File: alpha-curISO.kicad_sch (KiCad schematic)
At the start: 169 parts, among them SW1 SW_Push_45deg, SW10 SW_Push_45deg, SW11 SW_Push_45deg, SW11(2)1 SW_Push_45deg, SW12 SW_Push_45deg, SW13 SW_Push_45deg, SW14 SW_Push_45deg, SW15 SW_Push_45deg, SW16 SW_Push_45deg, SW17 SW_Push_45deg, SW18 SW_Push_45deg, SW19 SW_Push_45deg, SW2 SW_Push_45deg, SW20 SW_Push_45deg, SW21 SW_Push_45deg, SW22 SW_Push_45deg, SW22(1.5)1 SW_Push_45deg, SW23 SW_Push_45deg, SW23(1.5)1 SW_Push_45deg, SW24 SW_Push_45deg, SW24(2)1 SW_Push_45deg, SW24(ISO)1 SW_Push_45deg, SW25 SW_PUSH, SW25(1.25)1 SW_Push_45deg, SW25(1.5)1 SW_Push_45deg, SW25(ortho)1 SW_Push_45deg, SW26 SW_Push_45deg, SW26(ortho)1 SW_Push_45deg, SW27 SW_Push_45deg, SW27(ortho)1 SW_Push_45deg, SW28 SW_Push_45deg, SW28(ortho)1 SW_Push_45deg, SW29 SW_Push_45deg, SW29(ortho)1 SW_Push_45deg, SW3 SW_Push_45deg, SW30 SW_Push_45deg, SW30(ortho)1 SW_Push_45deg, SW31 SW_Push_45deg, SW31(ortho)1 SW_Push_45deg, SW32 SW_Push_45deg, SW32(ortho)1 SW_Push_45deg, SW33 SW_Push_45deg, SW33(ortho)1 SW_Push_45deg, SW34 SW_Push_45deg, SW34(ortho)1 SW_Push_45deg, SW35 SW_Push_45deg, SW35(ortho)1 SW_Push_45deg, SW36 SW_PUSH, SW36(1.25)1 SW_Push_45deg, SW36(1.5)1 SW_Push_45deg, SW36(ortho)1 SW_Push_45deg, SW37 SW_Push_45deg, SW37(1.5)1 SW_Push_45deg, SW38 SW_Push_45deg, SW38(3)1 SW_Push_45deg, SW39 SW_Push_45deg, SW39(1.5)1 SW_Push_45deg, SW4 SW_Push_45deg, SW40 SW_PUSH, SW40(1.25)1 SW_Push_45deg, SW40(1.5)1 SW_Push_45deg, SW40(3)1 SW_Push_45deg, SW41(1.75)1 SW_Push_45deg, SW41(1.75a)1 SW_Push_45deg, SW41(1.75a)2 SW_Push_45deg, SW41(2)1 SW_Push_45deg, SW41(2.25)1 SW_Push_45deg, SW42 SW_Push_45deg, SW42(3)1 SW_Push_45deg, SW42(6)1 SW_Push_45deg, SW43(1.75)1 SW_Push_45deg, SW43(2)1 SW_Push_45deg, SW43(2.25)1 SW_Push_45deg, SW44(1.25)1 SW_Push_45deg, SW44(1.5)1 SW_Push_45deg, SW44(3)1 SW_Push_45deg, SW45 SW_Push_45deg, SW45(1.5)1 SW_Push_45deg, SW46 SW_Push_45deg, SW46(3)1 SW_Push_45deg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

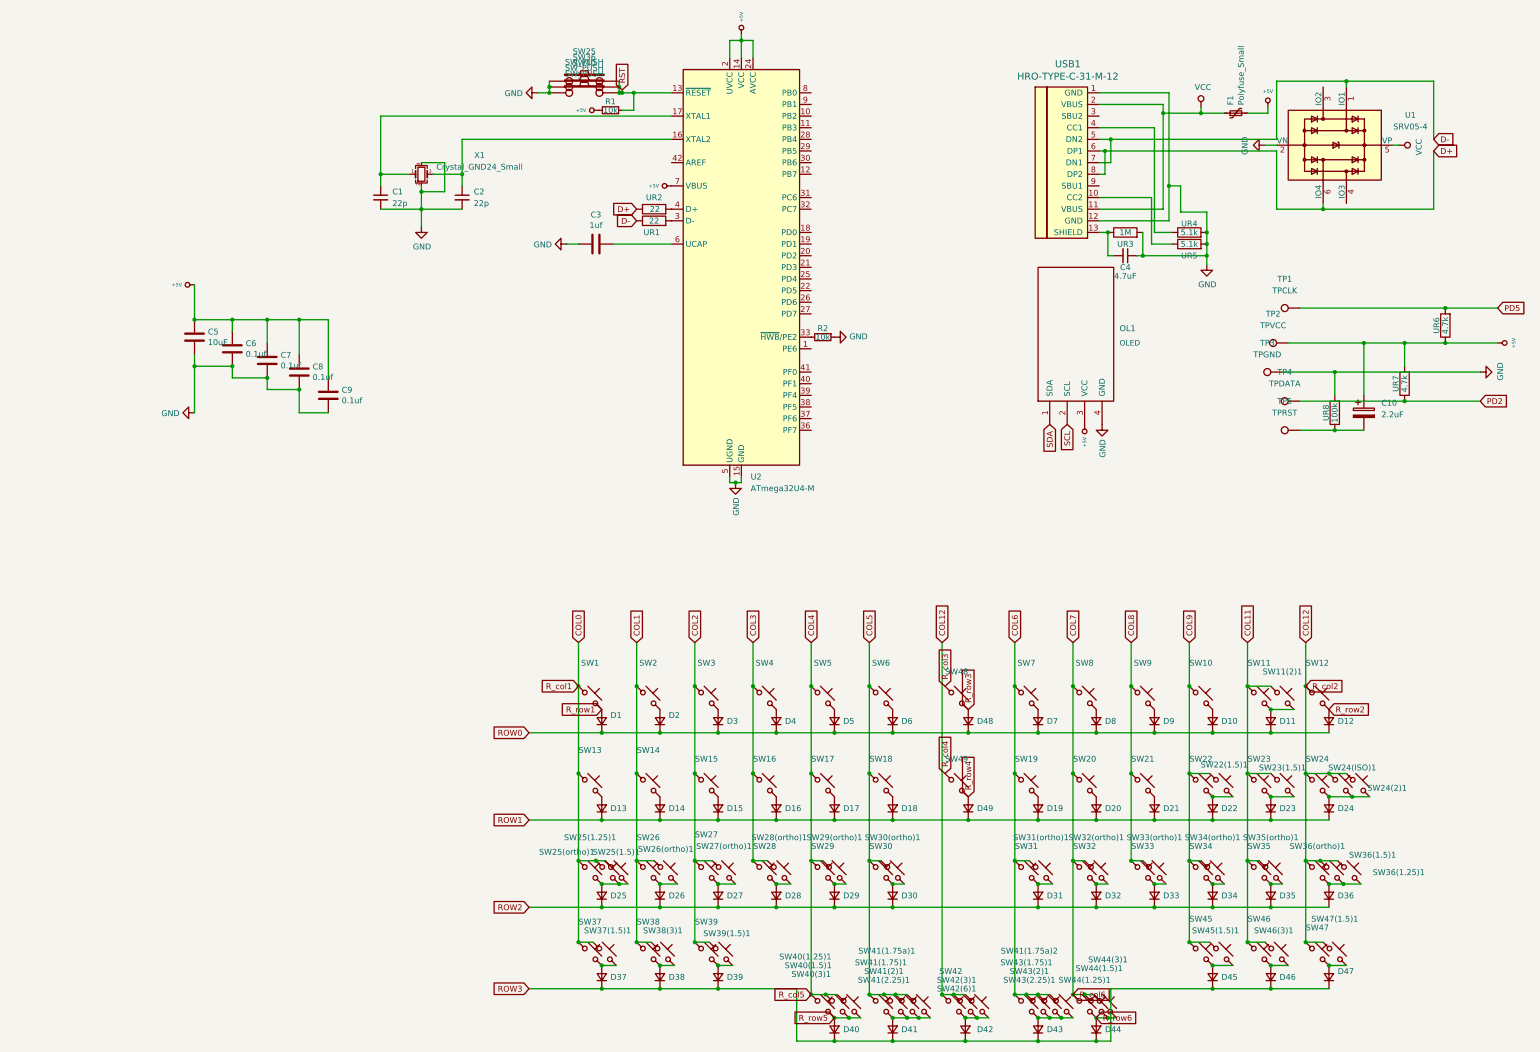
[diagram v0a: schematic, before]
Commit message: split schematics
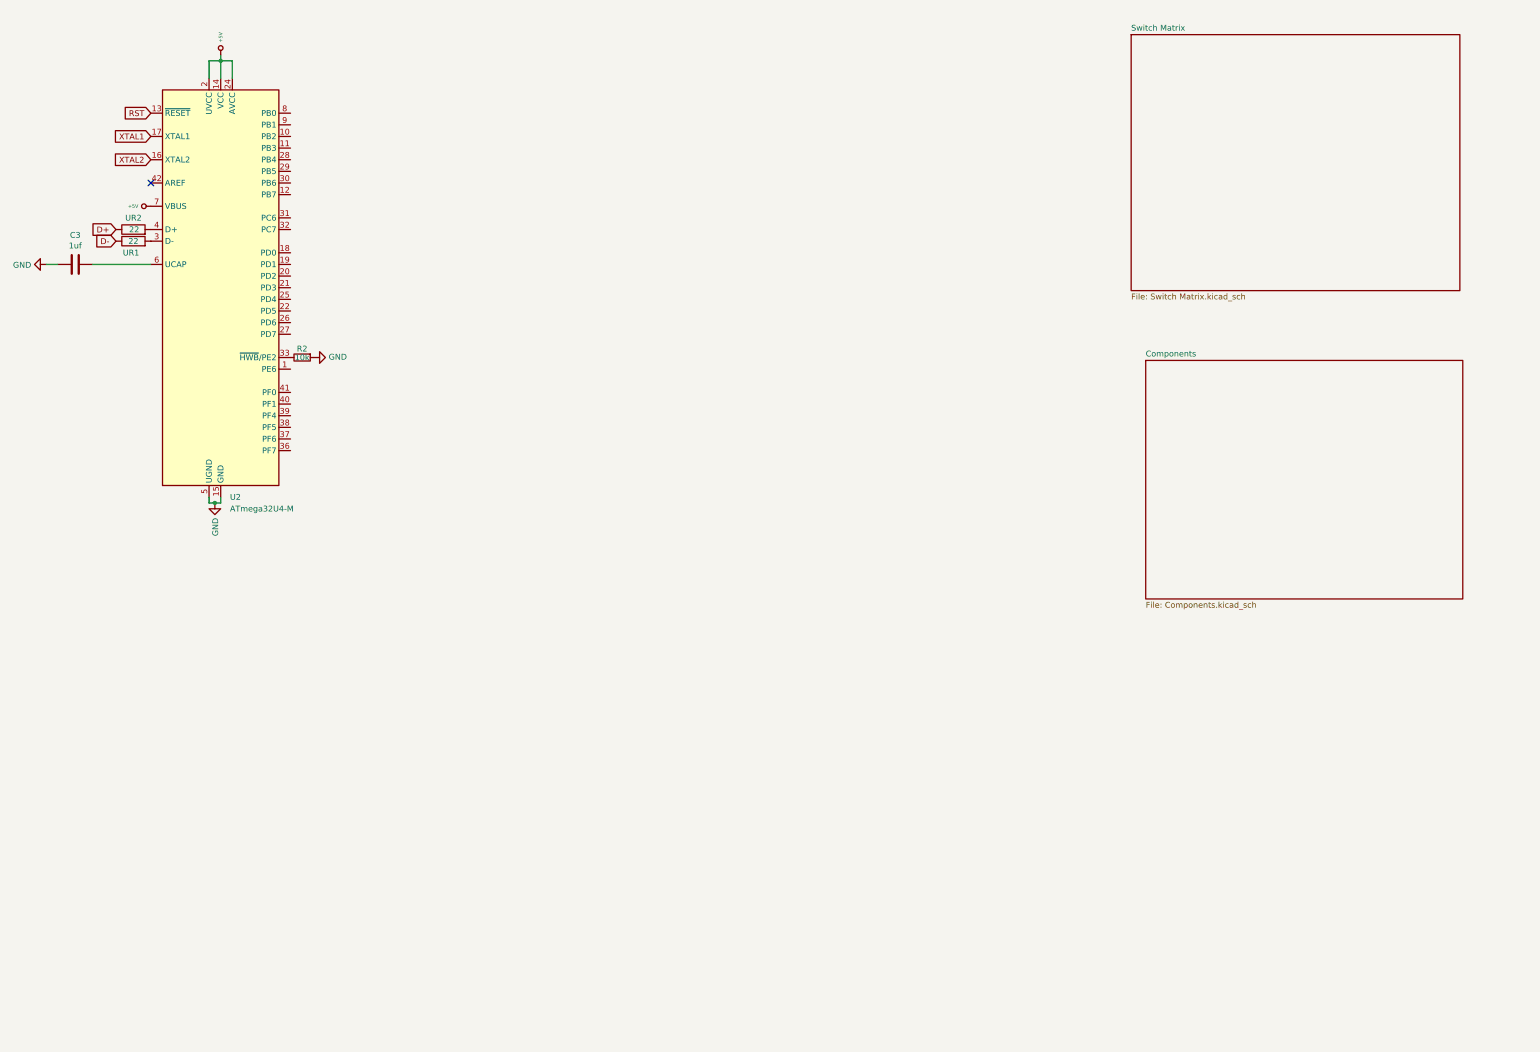
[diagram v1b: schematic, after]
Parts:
- removed C1, C2: 22p, Capacitor_SMD:C_0805_2012Metric, symbol Device:C_Small
- removed C10: 2.2uF, Capacitor_SMD:C_0805_2012Metric_Pad1.18x1.45mm_HandSolder, symbol Device:C_Polarized
- removed C4: 4.7uF, Capacitor_SMD:C_0805_2012Metric, symbol device:C_Small
- removed C5: 10uF, Capacitor_SMD:C_0805_2012Metric, symbol device:C
- removed C6, C7, C8, C9: 0.1uf, Capacitor_SMD:C_0805_2012Metric, symbol device:C
- removed D1, D10, D11, D12, D13, D14, D15, D16, D17, D18, D19, D2, D20, D21, D22, D23, D24, D25, D26, D27, D28, D29, D3, D30, D31, D32, D33, D34, D35, D36, D37, D38, D39, D4, D40, D41, D42, D43, D44, D45, D46, D47, D48, D49, D5, D6, D7, D8, D9: D_Small, symbol Device:D_Small
- removed F1: Polyfuse_Small, Fuse:Fuse_1206_3216Metric_Pad1.42x1.75mm_HandSolder, symbol device:Polyfuse_Small
- removed OL1: OLED, kbd:OLED_v2, symbol kbd:OLED
- removed R1: 10k, Resistor_SMD:R_0805_2012Metric, symbol device:R_Small
- removed SW1, SW10, SW11, SW11(2)1, SW12, SW13, SW14, SW15, SW16, SW17, SW18, SW19, SW2, SW20, SW21, SW22, SW22(1.5)1, SW23, SW23(1.5)1, SW24, SW24(2)1, SW24(ISO)1, SW25(1.25)1, SW25(1.5)1, SW25(ortho)1, SW26, SW26(ortho)1, SW27, SW27(ortho)1, SW28, SW28(ortho)1, SW29, SW29(ortho)1, SW3, SW30, SW30(ortho)1, SW31, SW31(ortho)1, SW32, SW32(ortho)1, SW33, SW33(ortho)1, SW34, SW34(ortho)1, SW35, SW35(ortho)1, SW36(1.25)1, SW36(1.5)1, SW36(ortho)1, SW37, SW37(1.5)1, SW38, SW38(3)1, SW39, SW39(1.5)1, SW4, SW40(1.25)1, SW40(1.5)1, SW40(3)1, SW41(1.75)1, SW41(1.75a)1, SW41(1.75a)2, SW41(2)1, SW41(2.25)1, SW42, SW42(3)1, SW42(6)1, SW43(1.75)1, SW43(2)1, SW43(2.25)1, SW44(1.25)1, SW44(1.5)1, SW44(3)1, SW45, SW45(1.5)1, SW46, SW46(3)1, SW47, SW47(1.5)1, SW48, SW49, SW5, SW6, SW7, SW8, SW9: SW_Push_45deg, symbol Switch:SW_Push_45deg
- removed SW25, SW40: SW_PUSH, Button_Switch_SMD:SW_SPST_SKQG_WithoutStem, symbol keyboard_parts:SW_PUSH
- removed SW36: SW_PUSH, Connector_PinHeader_2.54mm:PinHeader_1x02_P2.54mm_Vertical, symbol keyboard_parts:SW_PUSH
- removed TP1: TPCLK, TestPoint:TestPoint_THTPad_1.0x1.0mm_Drill0.5mm, symbol Connector:TestPoint
- removed TP2: TPVCC, TestPoint:TestPoint_THTPad_1.0x1.0mm_Drill0.5mm, symbol Connector:TestPoint
- removed TP3: TPGND, TestPoint:TestPoint_THTPad_1.0x1.0mm_Drill0.5mm, symbol Connector:TestPoint
- removed TP4: TPDATA, TestPoint:TestPoint_THTPad_1.0x1.0mm_Drill0.5mm, symbol Connector:TestPoint
- removed TP5: TPRST, TestPoint:TestPoint_THTPad_1.0x1.0mm_Drill0.5mm, symbol Connector:TestPoint
- removed U1: SRV05-4, Package_TO_SOT_SMD:SOT-23-6, symbol Power_Protection:SRV05-4
- removed UR3: 1M, Resistor_SMD:R_0805_2012Metric, symbol device:R
- removed UR4, UR5: 5.1k, Resistor_SMD:R_0805_2012Metric, symbol device:R
- removed UR6, UR7: 4.7k, Resistor_SMD:R_0805_2012Metric_Pad1.20x1.40mm_HandSolder, symbol device:R
- removed UR8: 100k, Resistor_SMD:R_0805_2012Metric_Pad1.20x1.40mm_HandSolder, symbol device:R
- removed USB1: HRO-TYPE-C-31-M-12, Type-C:HRO-TYPE-C-31-M-12-HandSoldering, symbol Type-C:HRO-TYPE-C-31-M-12
- removed X1: Crystal_GND24_Small, Crystal:Crystal_SMD_3225-4Pin_3.2x2.5mm_HandSoldering, symbol Device:Crystal_GND24_Small
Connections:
- net XTAL1: now reaches U2.17 (XTAL1)
- net XTAL2: now reaches U2.16 (XTAL2)
- no-connect marks 0 -> 1
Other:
- added sheet Components (Components.kicad_sch)
- added sheet Switch Matrix (Switch Matrix.kicad_sch)
- moved on the sheet: C3, R2, U2, UR1, UR2
